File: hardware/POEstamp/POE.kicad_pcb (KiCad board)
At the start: 2 copper layers, 70 x 40 mm, 61 parts, among them J1 0813-1X1T-57-F, P3 GND, P4 +5V, P5 CONN_01X05, P6 5Vout, P7 GNDout, Q1 SI3440DV, NFET, Q2 2N7002, Q3 MMBTA42, T1 PA1134, U1 LTC4267-3, U3 PS2811

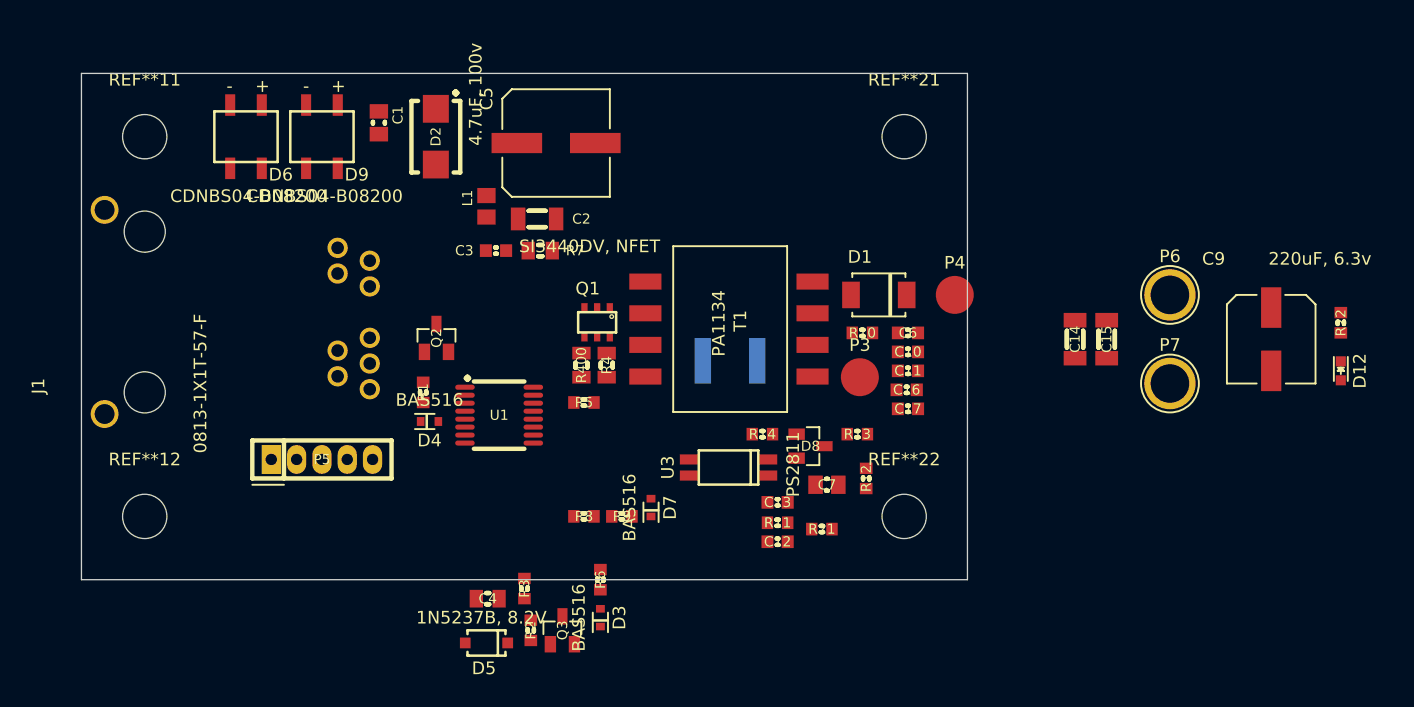
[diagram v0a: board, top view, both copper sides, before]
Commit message: Almost everything is in an OK spot on the PCB.
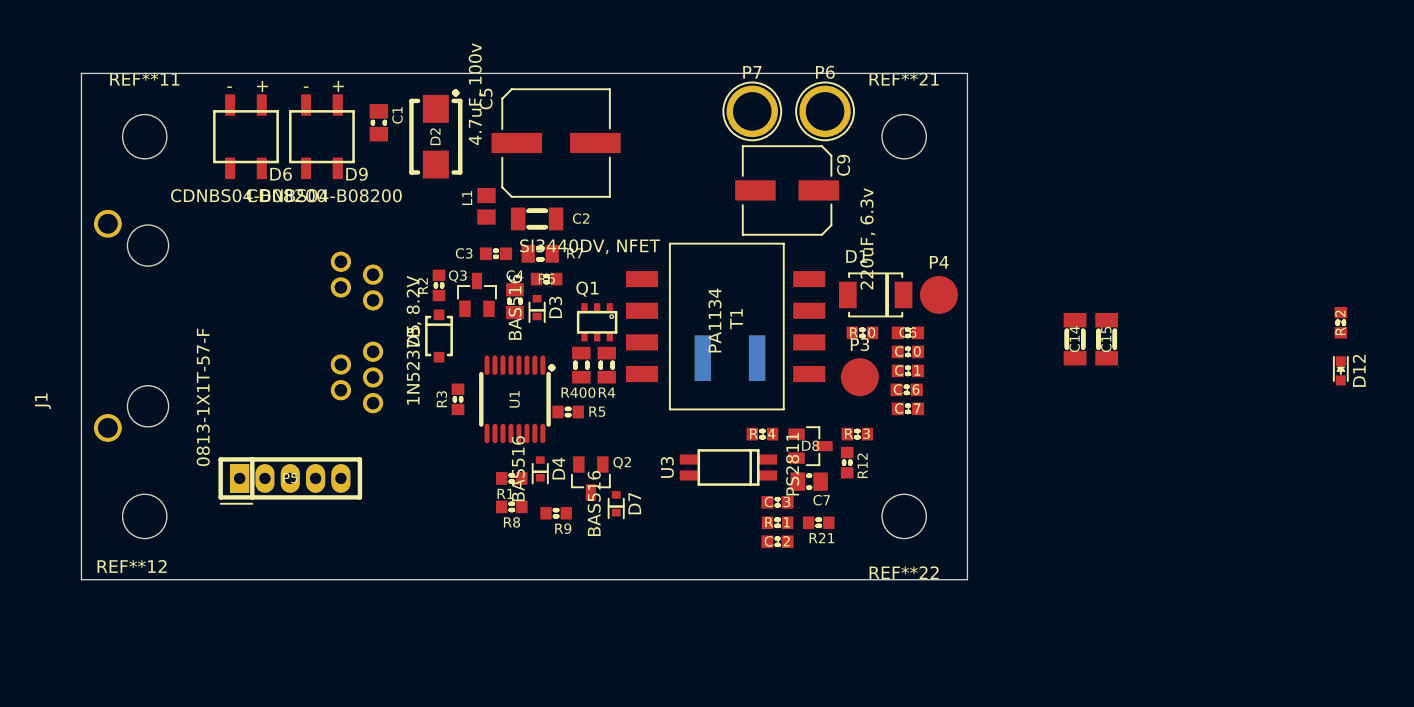
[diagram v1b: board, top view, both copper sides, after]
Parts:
- moved C9 40.0 mm to (125.8, 43.2), turned to 270 degrees
- moved P7 39.4 mm to (123.0, 37.0)
- moved P6 30.9 mm to (128.8, 37.0)
- moved R2 28.2 mm to (98.2, 50.8)
- moved Q3 27.3 mm to (101.2, 51.5)
- moved D3 25.0 mm to (106.0, 52.5)
- moved D5 24.5 mm to (98.2, 54.8), turned to 270 degrees
- moved R6 24.1 mm to (106.8, 50.2), turned to 0 degrees
- moved C4 23.6 mm to (104.2, 52.0), turned to 90 degrees
- moved Q2 16.5 mm to (110.2, 66.0), turned to 270 degrees
- moved R3 15.8 mm to (99.8, 59.8), turned to 90 degrees
- moved R1 9.76 mm to (104.0, 66.0), turned to 0 degrees
- moved D4 9.52 mm to (106.2, 65.2), turned to 270 degrees
- moved R8 5.75 mm to (104.0, 68.2)
- moved R9 5.21 mm to (107.5, 68.8)
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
